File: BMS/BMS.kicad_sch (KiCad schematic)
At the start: 43 parts, among them J1 Cell Taps, J2 Temp Sensors, J3 IsoSPI, J4 IsoSPI, Q1 NSV1C201MZ4, SW1 SW_DIP_x04, U1 LTC6811, U2 ADG708

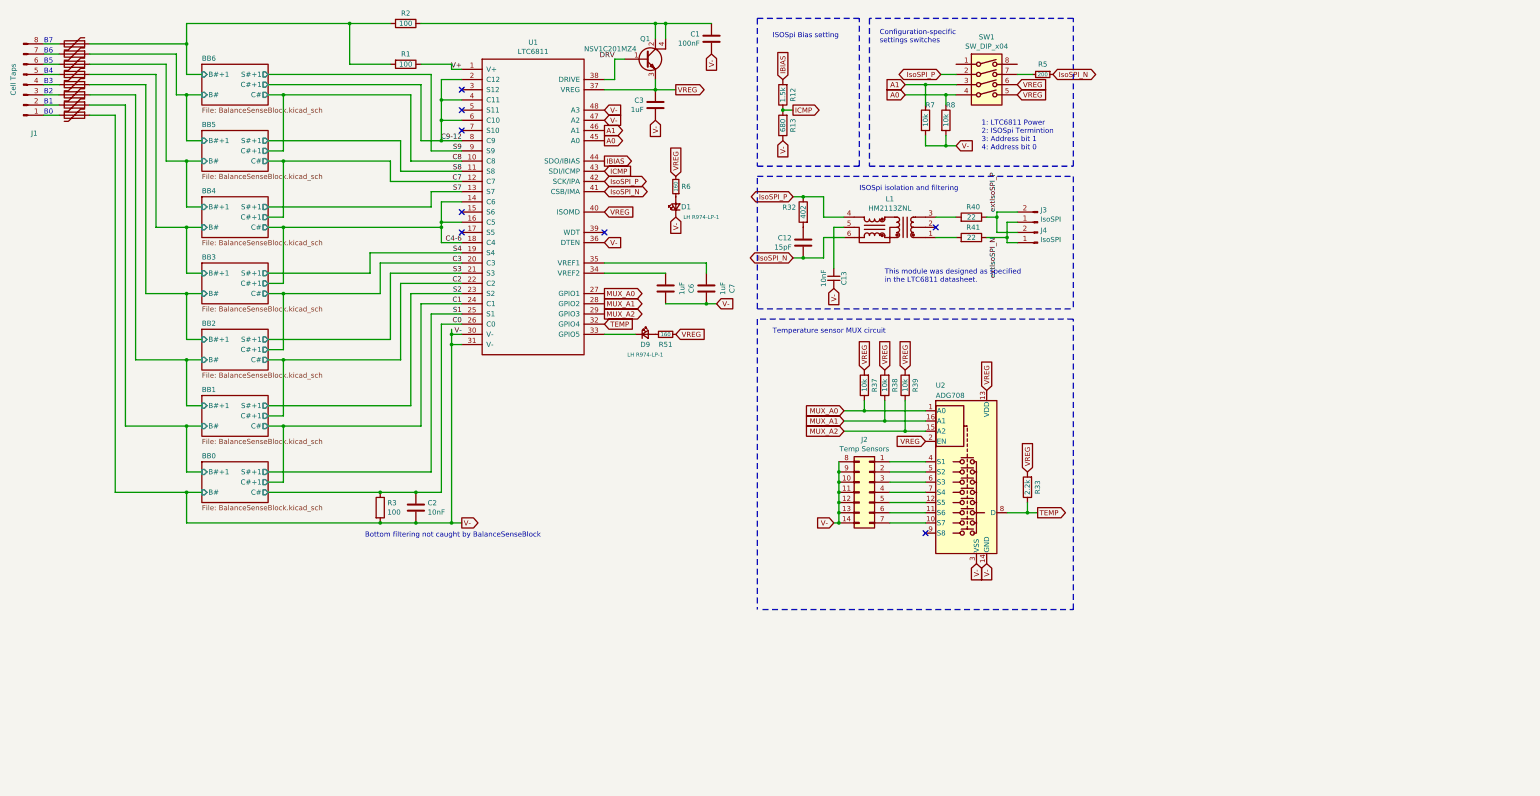
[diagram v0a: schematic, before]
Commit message: BMS Schema Done!
hello world
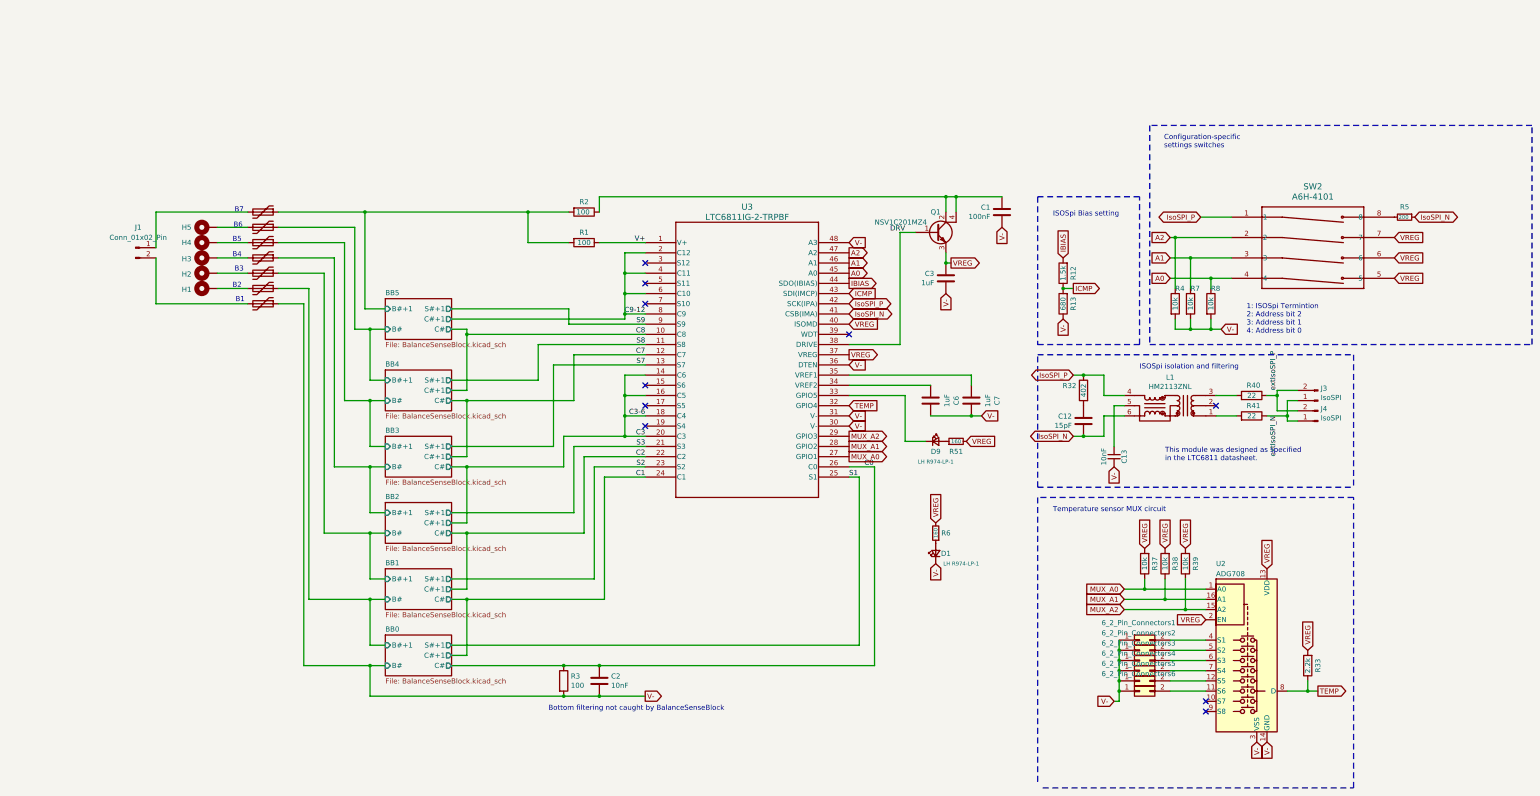
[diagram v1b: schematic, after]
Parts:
- removed F1: Polyfuse, Fuse:Fuse_1812_4532Metric_Pad1.30x3.40mm_HandSolder, symbol Device:Polyfuse
- removed J1: Cell Taps, Connector_Molex:Molex_Nano-Fit_105313-xx08_1x08_P2.50mm_Horizontal, symbol Connector:Conn_01x08_Pin
- removed J2: Temp Sensors, Connector_Molex:Molex_Nano-Fit_105314-xx14_2x07_P2.50mm_Horizontal, symbol Connector_Generic:Conn_02x07_Top_Bottom
- removed SW1: SW_DIP_x04, FSFootprints:DIP A6H-4101, symbol Switch:SW_DIP_x04
- removed U1: LTC6811, 1FS_2_Global_Footprint_Library:FSOP-48_[LTC6811-2], symbol FSSymbols:LTC6811
- added 6_2_Pin_Connectors1, 6_2_Pin_Connectors2, 6_2_Pin_Connectors3, 6_2_Pin_Connectors4, 6_2_Pin_Connectors5, 6_2_Pin_Connectors6: ~, Connector_Molex:Molex_Nano-Fit_105313-xx02_1x02_P2.50mm_Horizontal, symbol Connector_Generic:Conn_02x01
- added H1, H2, H3, H4, H5: MountingHole_Pad, MountingHole:MountingHole_3.2mm_M3_DIN965_Pad, symbol Mechanical:MountingHole_Pad
- added J1: Conn_01x02_Pin, Connector_Molex:Molex_Nano-Fit_105313-xx02_1x02_P2.50mm_Horizontal, symbol Connector:Conn_01x02_Pin
- added R4: 10k, Resistor_SMD:R_0805_2012Metric_Pad1.20x1.40mm_HandSolder, symbol Device:R
- added SW2: A6H-4101, FS_3_Global_Footprint_Library:SW_A6H-4101_OMR, symbol FS_3_Global_Symbol_Library:A6H-4101
- added U3: LTC6811IG-2-TRPBF, FS_3_Global_Footprint_Library:LTC6811-2, symbol FS_3_Global_Symbol_Library:LTC6811IG-2-TRPBF
- C1, C12, C13, C2, C3, C6, C7, R3: footprint Capacitor_SMD:C_0805_2012Metric_Pad1.15x1.40mm_HandSolder -> Capacitor_SMD:C_0805_2012Metric_Pad1.18x1.45mm_HandSolder
- L1: footprint FSFootprints:HM2113ZNL -> FS_3_Global_Footprint_Library:HM2113ZNLT
- R1, R12, R13, R2, R32, R33, R37, R38, R39, R40, R41, R5, R51, R6, R7, R8: footprint Resistor_SMD:R_0805_2012Metric_Pad1.15x1.40mm_HandSolder -> Resistor_SMD:R_0805_2012Metric_Pad1.20x1.40mm_HandSolder
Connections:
- net BB6/B#+1 is gone; now on net BB5/B#+1: R1.2, R2.2
- net A0: now also SW2.4, U3.45 (A0)
- net A1: now also SW2.3, U3.46 (A1)
- net C0: now also U3.26 (C0)
- net C1: now also U3.24 (C1)
- net C2: now also U3.22 (C2)
- net C3: now also U3.14 (C6), U3.16 (C5), U3.18 (C4), U3.20 (C3)
- net C7: now also U3.12 (C7)
- net C8: now also U3.10 (C8)
- net C9-12: now also U3.2 (C12), U3.4 (C11), U3.6 (C10), U3.8 (C9)
- net DRV: now also U3.38 (DRIVE)
- net IBIAS: now also U3.44 (SDO(IBIAS))
- net ICMP: now also U3.43 (SDI(IMCP))
- net IsoSPI_N: now also U3.41 (CSB(IMA))
- net IsoSPI_P: now also SW2.1, U3.42 (SCK(IPA))
- net MUX_A0: now also U3.27 (GPIO1)
- net MUX_A1: now also U3.28 (GPIO2)
- net MUX_A2: now also U3.29 (GPIO3)
- net S1: now also U3.25 (S1)
- net S2: now also U3.23 (S2)
- net S3: now also U3.21 (S3)
- net S7: now also U3.13 (S7)
- net S8: now also U3.11 (S8)
- net S9: now also U3.9 (S9)
- net TEMP: now also U3.32 (GPIO4)
- net V+: now also U3.1 (V+)
- net V-: now also 6_2_Pin_Connectors1.1 (Pin_1), 6_2_Pin_Connectors2.1 (Pin_1), 6_2_Pin_Connectors3.1 (Pin_1), 6_2_Pin_Connectors4.1 (Pin_1), 6_2_Pin_Connectors5.1 (Pin_1), 6_2_Pin_Connectors6.1 (Pin_1), R4.2, U3.30 (V-), U3.31 (V-), U3.36 (DTEN), U3.48 (A3)
- net VREG: now also SW2.5, SW2.6, SW2.7, U3.37 (VREG), U3.40 (ISOMD)
- net at D9.1 (K): now also U3.33 (GPIO5)
- net at C6.2: now also U3.34 (VREF2)
- net at C7.2: now also U3.35 (VREF1)
- net at F8.2: now also J1.2 (Pin_2)
- net at F7.2: now also H1.1
- net at F6.2: now also H2.1
- net at F5.2: now also H3.1
- net at F4.2: now also H4.1
- net at F3.2: now also H5.1
- net at F2.2: now also J1.1 (Pin_1)
- net at R5.2: now also SW2.8
- net at U2.11 (S6): now also 6_2_Pin_Connectors6.2 (Pin_2)
- net at U2.12 (S5): now also 6_2_Pin_Connectors5.2 (Pin_2)
- net at U2.4 (S1): now also 6_2_Pin_Connectors1.2 (Pin_2)
- net at U2.5 (S2): now also 6_2_Pin_Connectors2.2 (Pin_2)
- net at U2.6 (S3): now also 6_2_Pin_Connectors3.2 (Pin_2)
- net at U2.7 (S4): now also 6_2_Pin_Connectors4.2 (Pin_2)
- new net A2: R4.1, SW2.2, U3.47 (A2)
- no-connect marks 8 -> 10
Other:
- removed sheet BB6
- note added: "1: ISOSpi Termintion 2: Address bit 2 3: Address bit 1 4: Address bit 0"
- note removed: "1: LTC6811 Power 2: ISOSpi Termintion 3: Address bit 1 4: Address bit 0"
- note removed: "B0"
- moved on the sheet: C1, C12, C13, C2, C3, C6, C7, D1, D9, J3, J4, L1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
